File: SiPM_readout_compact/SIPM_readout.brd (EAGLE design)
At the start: 50 x 25 mm, 26 parts

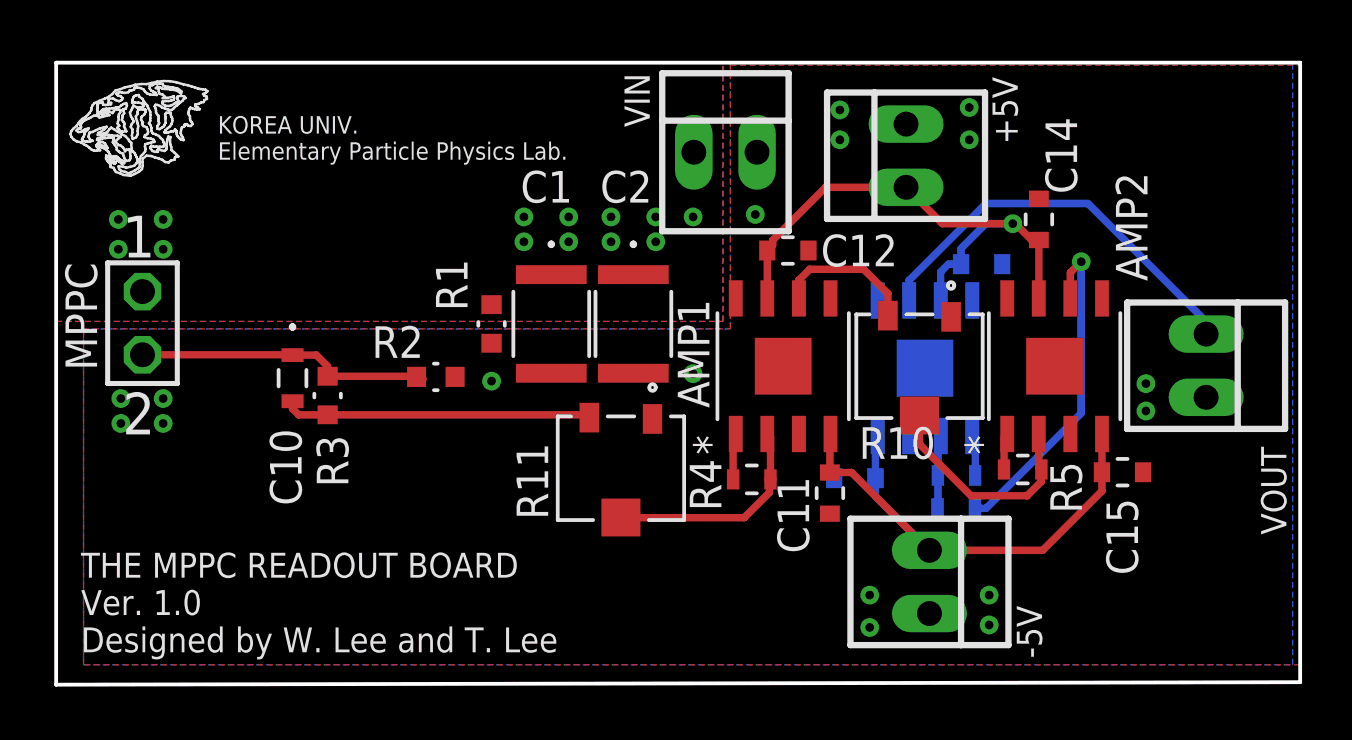
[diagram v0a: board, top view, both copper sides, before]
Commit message: HV
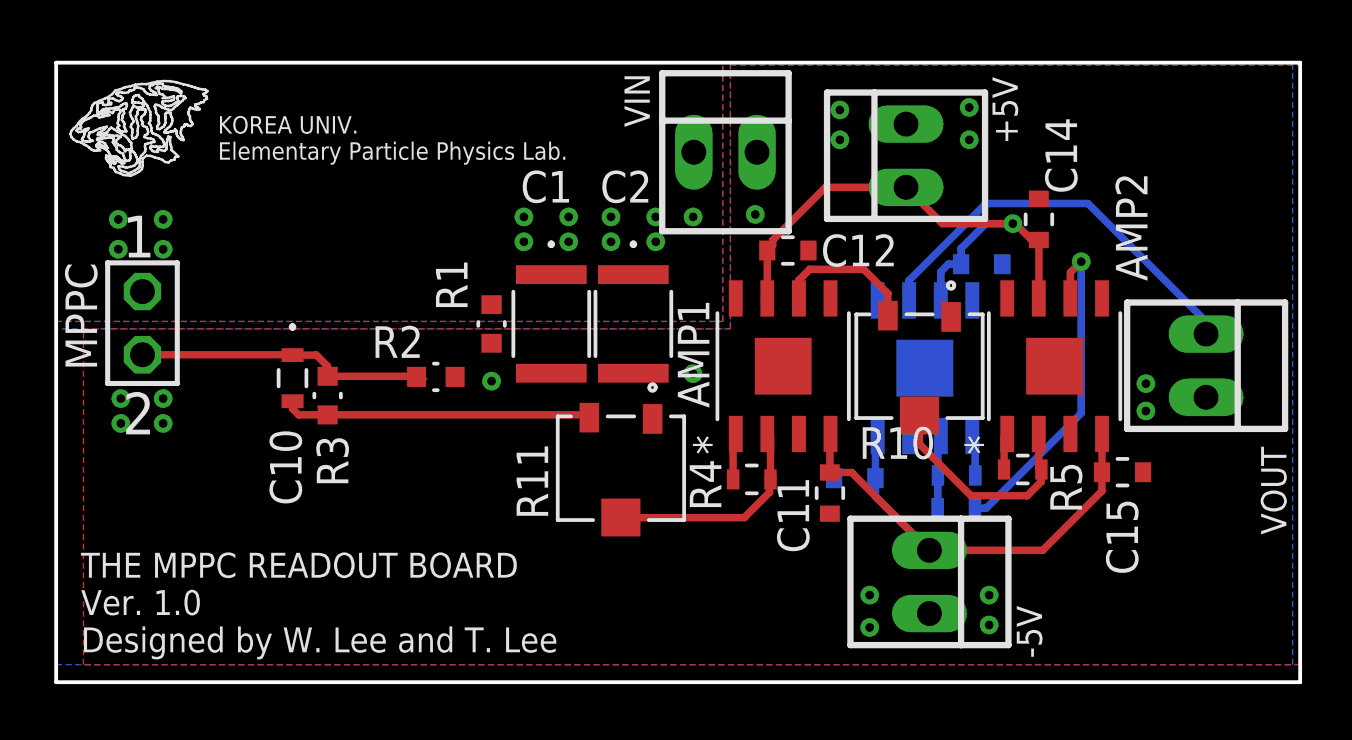
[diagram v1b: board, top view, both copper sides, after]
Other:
- board size 50 x 25 mm -> 50 x 24.9 mm
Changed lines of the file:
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@@
 <layer number="14" name="Route14" color="22" fill="1" visible="no" active="no"/>
 <layer number="15" name="Route15" color="23" fill="1" visible="no" active="no"/>
-<layer number="16" name="Bottom" color="1" fill="1" visible="yes" active="yes"/>
+<layer number="16" name="Bottom" color="1" fill="1" visible="no" active="yes"/>
 <layer number="17" name="Pads" color="2" fill="1" visible="yes" active="yes"/>
 <layer number="18" name="Vias" color="2" fill="1" visible="yes" active="yes"/>
@@
 <layer number="20" name="Dimension" color="24" fill="1" visible="yes" active="yes"/>
 <layer number="21" name="tPlace" color="7" fill="1" visible="yes" active="yes"/>
-<layer number="22" name="bPlace" color="7" fill="1" visible="yes" active="yes"/>
+<layer number="22" name="bPlace" color="7" fill="1" visible="no" active="yes"/>
 <layer number="23" name="tOrigins" color="15" fill="1" visible="yes" active="yes"/>
-<layer number="24" name="bOrigins" color="15" fill="1" visible="yes" active="yes"/>
+<layer number="24" name="bOrigins" color="15" fill="1" visible="no" active="yes"/>
 <layer number="25" name="tNames" color="7" fill="1" visible="yes" active="yes"/>
-<layer number="26" name="bNames" color="7" fill="1" visible="yes" active="yes"/>
+<layer number="26" name="bNames" color="7" fill="1" visible="no" active="yes"/>
 <layer number="27" name="tValues" color="7" fill="1" visible="no" active="yes"/>
 <layer number="28" name="bValues" color="7" fill="1" visible="no" active="yes"/>
@@
 <layer number="38" name="bTest" color="7" fill="1" visible="no" active="yes"/>
 <layer number="39" name="tKeepout" color="4" fill="11" visible="yes" active="yes"/>
-<layer number="40" name="bKeepout" color="1" fill="11" visible="yes" active="yes"/>
+<layer number="40" name="bKeepout" color="1" fill="11" visible="no" active="yes"/>
 <layer number="41" name="tRestrict" color="4" fill="10" visible="yes" active="yes"/>
-<layer number="42" name="bRestrict" color="1" fill="10" visible="yes" active="yes"/>
+<layer number="42" name="bRestrict" color="1" fill="10" visible="no" active="yes"/>
 <layer number="43" name="vRestrict" color="2" fill="10" visible="no" active="yes"/>
 <layer number="44" name="Drills" color="7" fill="1" visible="no" active="yes"/>
@@
 <layer number="50" name="dxf" color="7" fill="1" visible="no" active="no"/>
 <layer number="51" name="tDocu" color="7" fill="1" visible="yes" active="yes"/>
-<layer number="52" name="bDocu" color="7" fill="1" visible="yes" active="yes"/>
+<layer number="52" name="bDocu" color="7" fill="1" visible="no" active="yes"/>
 <layer number="53" name="tGND_GNDA" color="7" fill="1" visible="no" active="no"/>
 <layer number="54" name="bGND_GNDA" color="7" fill="1" visible="no" active="no"/>
@@
 <fusionsync huburn="a.cGVyc29uYWw6dWUyOWYzNGEwMQ" projecturn="a.cGVyc29uYWw6dWUyOWYzNGEwMSMyMDIxMDYxNjQyMDk2OTI1Ng" f3durn="urn:adsk.wipprod:dm.lineage:73l8zhv5RF-XBDXu35YORA" pcbguid="" lastpulledtime="" lastsyncedchangeguid="" latestrevisionid="a99baacc-6fba-49c1-9e69-8d64e022b22a" lastsyncedrevisionid="a99baacc-6fba-49c1-9e69-8d64e022b22a" lastboardhashguid="9c3b8375-83c7-0d3a-68b5-104893922fa0" lastpushedtime="2021-06-17T01:39:31Z" linktopcb3d="true"/>
 <plain>
-<wire x1="60.3" y1="64.8" x2="10.3" y2="64.7" width="0.1524" layer="20"/>
-<wire x1="10.3" y1="64.7" x2="10.3" y2="89.7" width="0.1524" layer="20"/>
+<wire x1="60.3" y1="64.8" x2="10.3" y2="64.8" width="0.1524" layer="20"/>
+<wire x1="10.3" y1="64.8" x2="10.3" y2="89.7" width="0.1524" layer="20"/>
 <wire x1="10.3" y1="89.7" x2="60.3" y2="89.7" width="0.1524" layer="20"/>
 <wire x1="60.3" y1="89.7" x2="60.3" y2="64.8" width="0.1524" layer="20"/>
@@
 <wire x1="15.86913125" y1="88.70725" x2="15.97313125" y2="88.67125" width="0.1" layer="25"/>
 <wire x1="15.97313125" y1="88.67125" x2="16.07313125" y2="88.64225" width="0.1" layer="25"/>
-<dimension x1="10.3" y1="89.7" x2="60.3" y2="89.7" x3="35.3" y3="94.3" textsize="1.778" layer="20"/>
 </plain>
 <attributes>
@@
 <contactref element="R10" pad="1"/>
 <polygon width="0.1" layer="16">
-<vertex x="11.4" y="65.5"/>
+<vertex x="10.3" y="65.5"/>
 <vertex x="60" y="65.5"/>
 <vertex x="60" y="89.69"/>
 <vertex x="37.4" y="89.69995625"/>
 <vertex x="37.4" y="79"/>
-<vertex x="11.4" y="79"/>
+<vertex x="10.3" y="79"/>
 </polygon>
 <contactref element="C11" pad="2"/>
